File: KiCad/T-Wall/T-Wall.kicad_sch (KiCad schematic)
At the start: 38 parts, among them J1 Conn_1, J2 Conn_2, J3 Conn_3, J4 Conn_4, J5 Conn_5, J6 Conn_6, J7 Conn_7, J8 Conn_8, J9 2086-1203_700-000_997-605, U1 TCA9555DBR, U2 SN74AHCT125N, U3 ESP32-S3-DevKitC, U4 TCA9555DBR, U5 TCA9555DBR, U6 TCA9555DBR

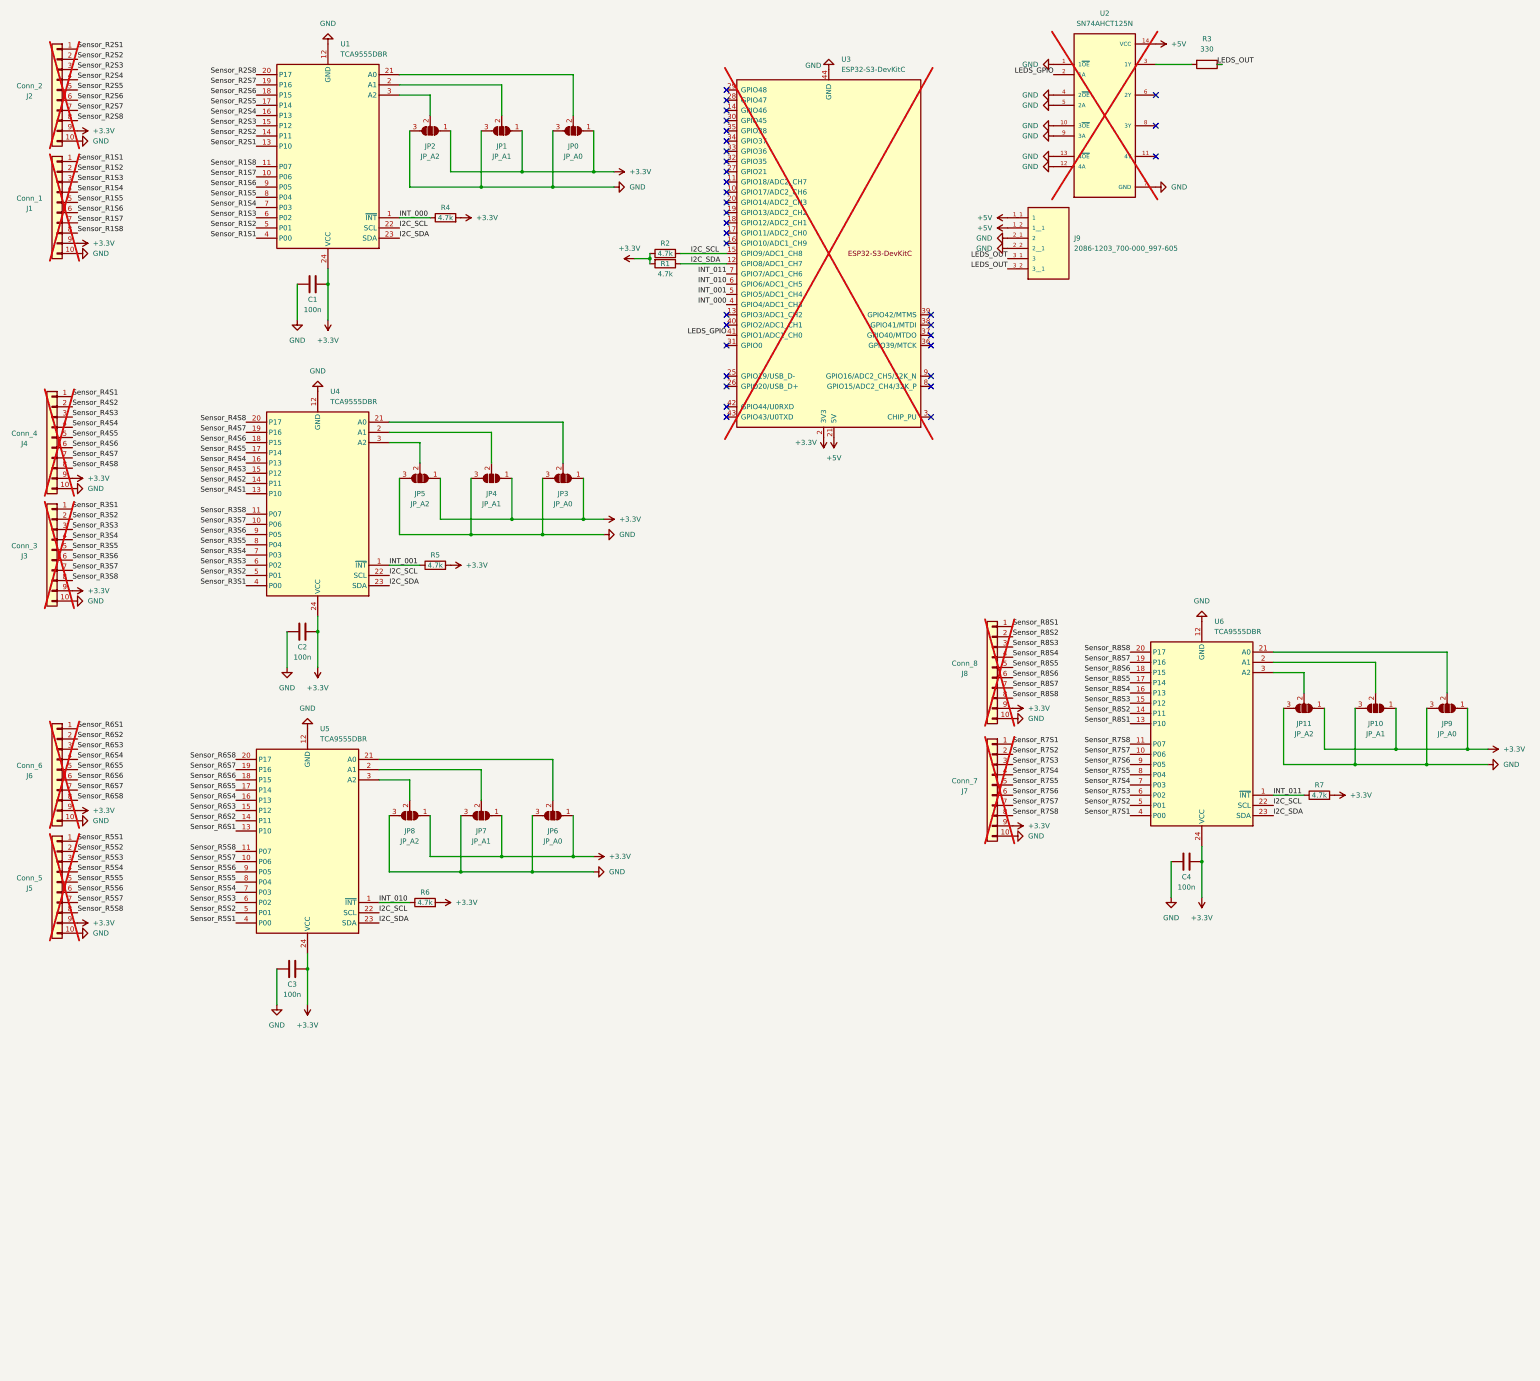
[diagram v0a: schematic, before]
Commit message: EOD 1303
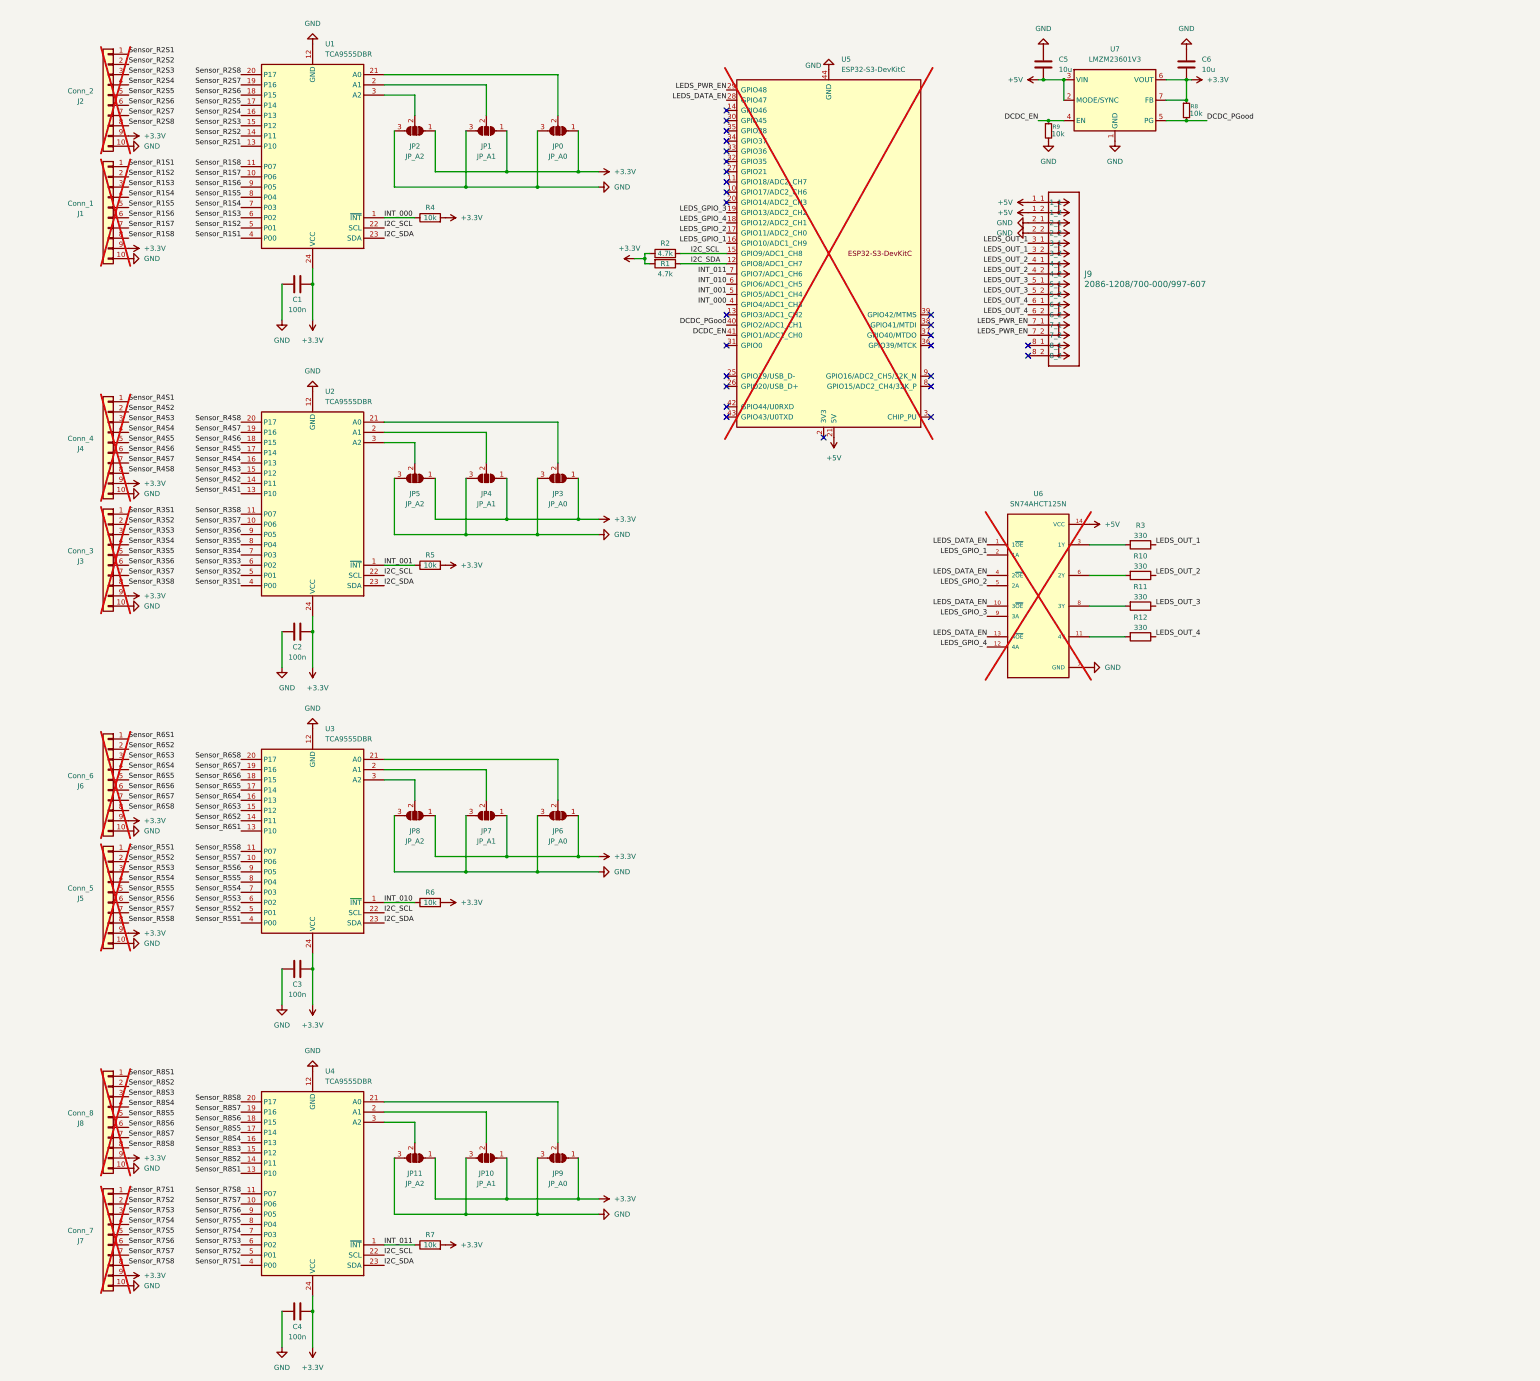
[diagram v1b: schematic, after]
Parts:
- removed J9: 2086-1203_700-000_997-605, 2086-1203_700-000_997-605:WAGO_2086-1203_700-000_997-605, symbol 2086-1203_700-000_997-605:2086-1203_700-000_997-605
- added C5, C6: 10u, Capacitor_SMD:C_1206_3216Metric_Pad1.33x1.80mm_HandSolder, symbol Device:C
- added J9: 2086-1208/700-000/997-607, 2086-1208_700-000_997-607:2086-1208_700-000_997-607, symbol 2068-1208_700-000_997-607:2086-1208_700-000_997-607
- added R10, R11, R12: 330, Resistor_SMD:R_0402_1005Metric_Pad0.72x0.64mm_HandSolder, symbol Device:R
- added R8, R9: 10k, Resistor_SMD:R_0402_1005Metric_Pad0.72x0.64mm_HandSolder, symbol Device:R_Small
- added U7: LMZM23601V3, Package_LGA:Texas_SIL0010A_MicroSiP-10-1EP_3.8x3mm_P0.6mm_EP0.7x2.9mm_ThermalVias, symbol Regulator_Switching:LMZM23601V3
- C1, C2, C3, C4: footprint Capacitor_SMD:C_0402_1005Metric -> Capacitor_SMD:C_0402_1005Metric_Pad0.74x0.62mm_HandSolder
- R1, R2, R3: footprint Resistor_SMD:R_0402_1005Metric -> Resistor_SMD:R_0402_1005Metric_Pad0.72x0.64mm_HandSolder
- R4, R5, R6, R7: value 4.7k -> 10k; footprint Resistor_SMD:R_0402_1005Metric -> Resistor_SMD:R_0402_1005Metric_Pad0.72x0.64mm_HandSolder; LCSC C25900 -> C25744
- renumbered U4 to U2, U5 to U3, U6 to U4, U3 to U5, U2 to U6
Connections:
- net +3.3V: now also C6.2, R8.1, U7.6 (VOUT), U7.7 (FB); no longer U5.1 (3V3), U5.2 (3V3)
- net +5V: now also C5.2, J9.1_1, J9.1_2, U7.2 (MODE/SYNC), U7.3 (VIN)
- net GND: now also C5.1, C6.1, J9.2_1, J9.2_2, R9.2, U7.1 (GND), U7.11 (GND); no longer U6.1 (1~{OE}), U6.10 (3~{OE}), U6.12 (4A), U6.13 (4~{OE}), U6.4 (2~{OE}), U6.5 (2A), U6.9 (3A)
- net at U6.11 (4Y): now also R12.2
- net at U6.6 (2Y): now also R10.2
- net at U6.8 (3Y): now also R11.2
- net LEDS_GPIO_1: now reaches U5.16 (GPIO10/ADC1_CH9)
- net LEDS_GPIO_1: now also U6.2 (1A)
- net LEDS_GPIO_2: now reaches U5.17 (GPIO11/ADC2_CH0)
- net LEDS_GPIO_2: now also U6.5 (2A)
- net LEDS_GPIO_4: now reaches U5.18 (GPIO12/ADC2_CH1)
- net LEDS_GPIO_4: now also U6.12 (4A)
- net LEDS_GPIO_3: now reaches U5.19 (GPIO13/ADC2_CH2)
- net LEDS_GPIO_3: now also U6.9 (3A)
- net LEDS_DATA_EN: now reaches U5.28 (GPIO47)
- net LEDS_DATA_EN: now also U6.1 (1~{OE}), U6.10 (3~{OE}), U6.13 (4~{OE}), U6.4 (2~{OE})
- net LEDS_PWR_EN: now reaches U5.29 (GPIO48)
- net LEDS_PWR_EN: now also J9.7_1, J9.7_2
- net DCDC_PGood: now reaches U5.40 (GPIO2/ADC1_CH1)
- net DCDC_PGood: now also R8.2, U7.5 (PG)
- net LEDS_GPIO renamed DCDC_EN
- net DCDC_EN: now also R9.1, U7.4 (EN); no longer U6.2 (1A)
- net LEDS_OUT renamed LEDS_OUT_1
- net LEDS_OUT_1: now also J9.3_1, J9.3_2
- new net: U5.1 (3V3), U5.2 (3V3)
- new net LEDS_OUT_2: J9.4_1, J9.4_2, R10.1
- new net LEDS_OUT_3: J9.5_1, J9.5_2, R11.1
- new net LEDS_OUT_4: J9.6_1, J9.6_2, R12.1
- no-connect marks 33 -> 26
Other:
- moved on the sheet: C1, C2, C3, C4, J1, J2, J3, J4, J5, J6, J7, J8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
